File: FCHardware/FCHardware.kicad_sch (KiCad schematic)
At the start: 26 parts, among them Q1 BUT11, U1 ESC_Xrotor_65A_4in1, U2 ESP32-S3-MINI-1U, U4 TPS629203, U5 MPU-6050

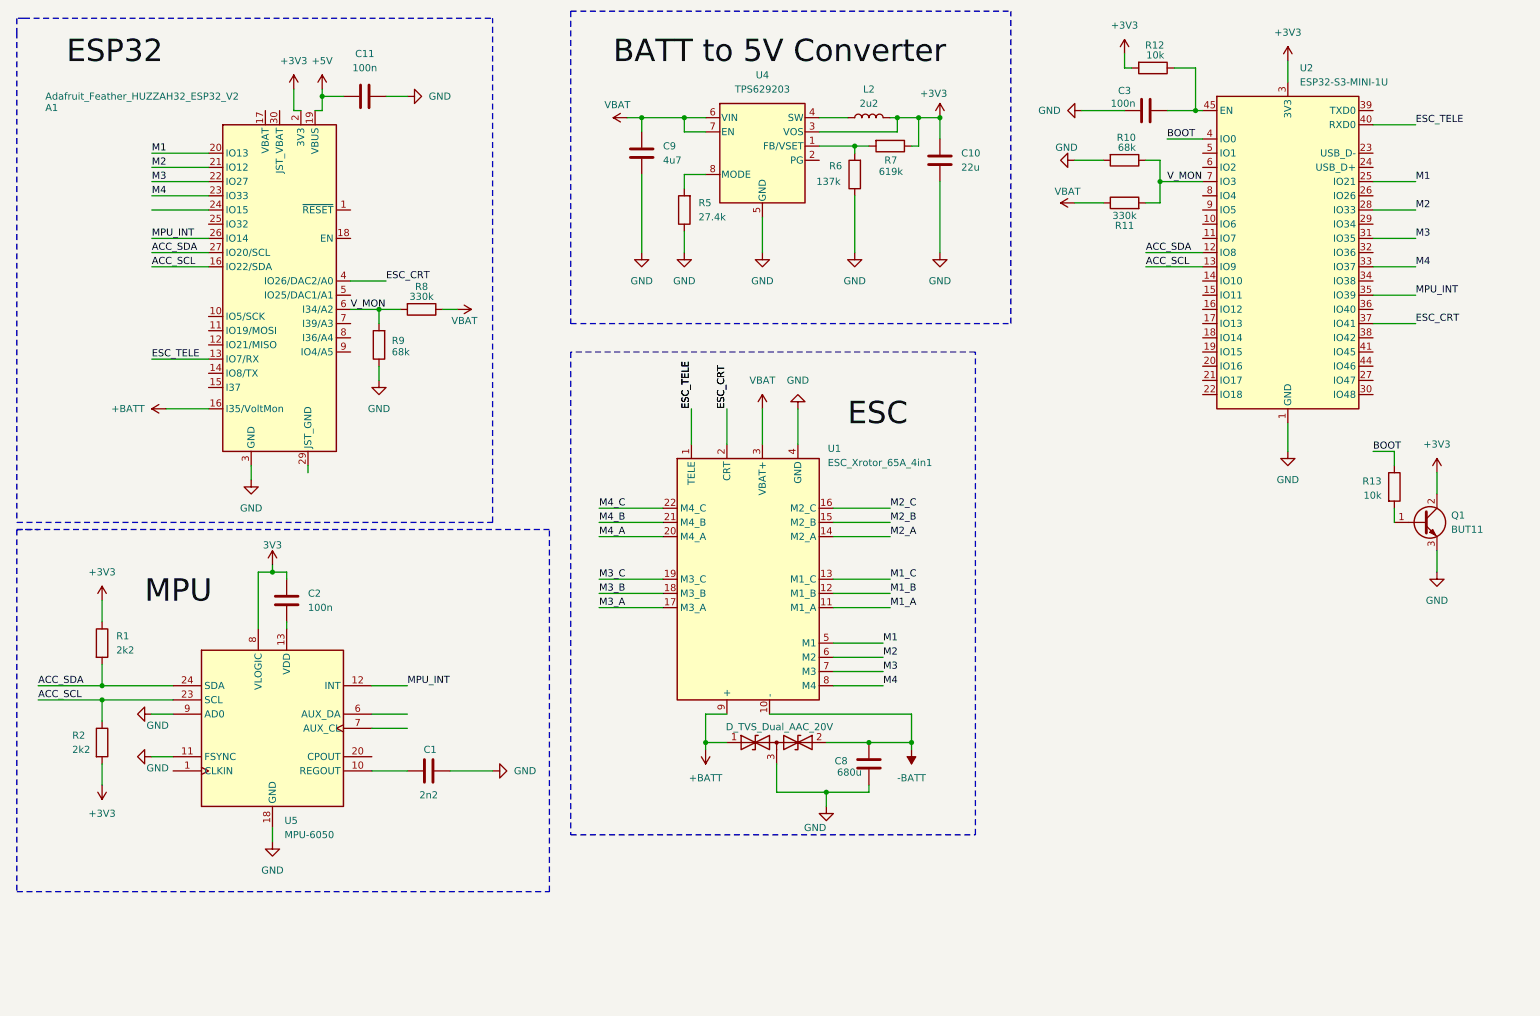
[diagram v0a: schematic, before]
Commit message: Final fixes before updating to 6S
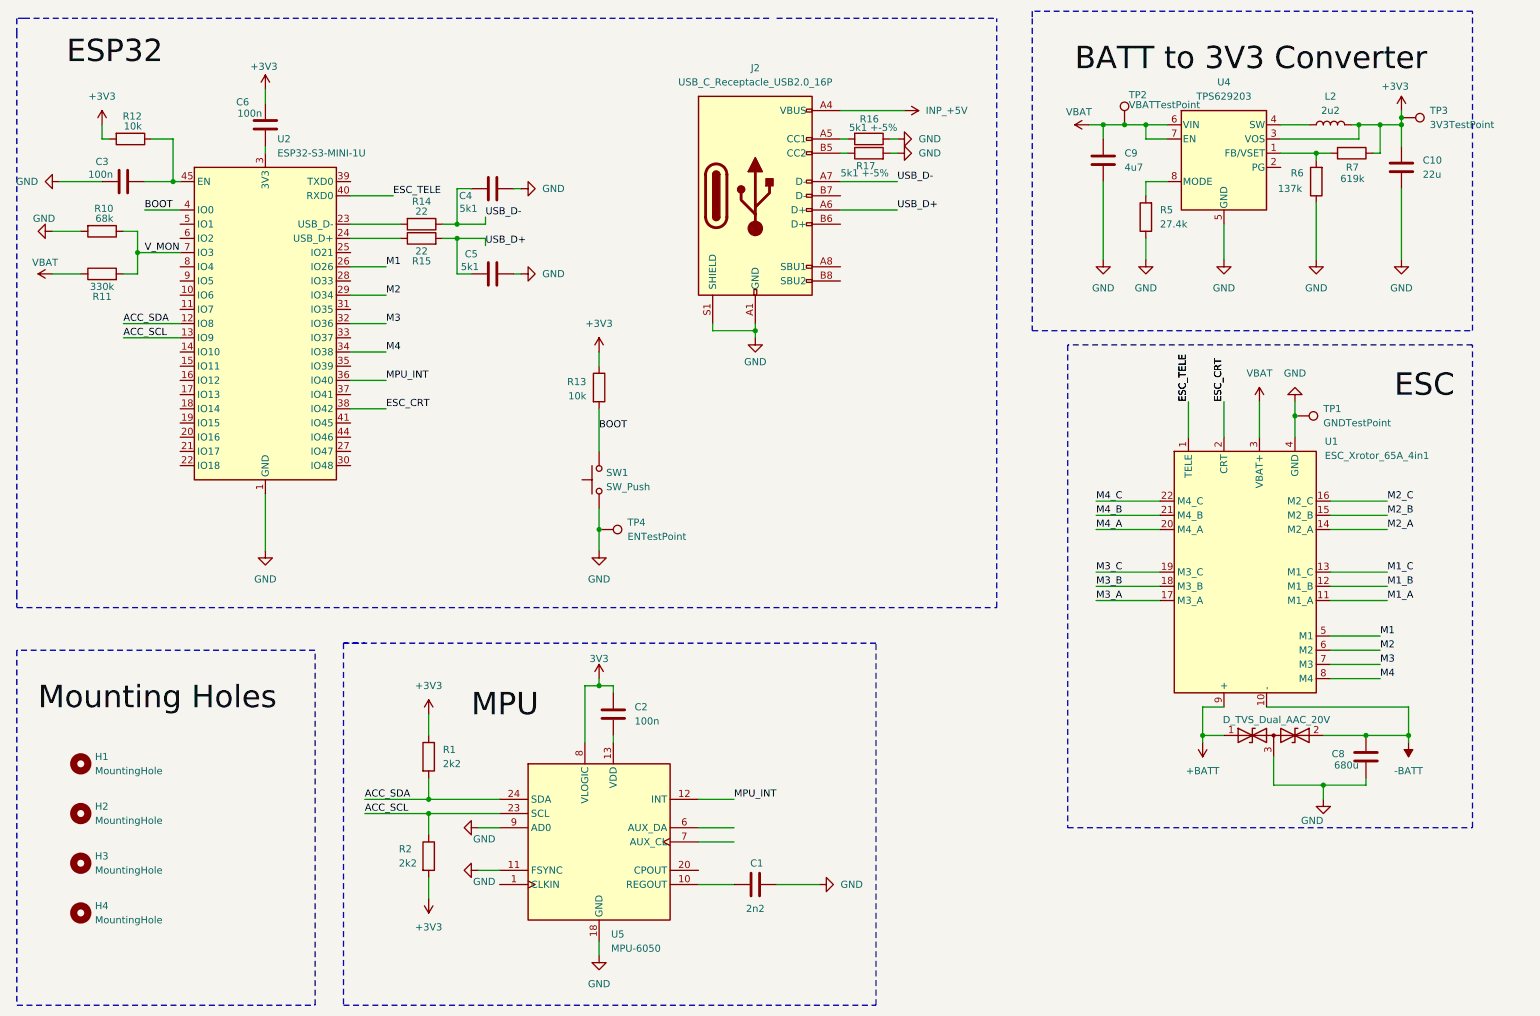
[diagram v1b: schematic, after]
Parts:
- removed A1: Adafruit_Feather_HUZZAH32_ESP32_V2, Module:Adafruit_Feather, symbol Custom_ESP32_Library:Adafruit_Feather_HUZZAH32_ESP32_v2
- removed C11: 100n, symbol Device:C
- removed Q1: BUT11, Package_TO_SOT_THT:TO-220-3_Vertical, symbol Transistor_BJT:BUT11
- removed R8: 330k, symbol Device:R
- removed R9: 68k, symbol Device:R
- added C4, C5: 5k1, symbol Device:C
- added C6: 100n, symbol Device:C
- added H1, H2, H3, H4: MountingHole, symbol Mechanical:MountingHole
- added J2: USB_C_Receptacle_USB2.0_16P, symbol Connector:USB_C_Receptacle_USB2.0_16P
- added R14, R15: 22, symbol Device:R
- added R16, R17: 5k1 +-5%, symbol Device:R
- added SW1: SW_Push, symbol Switch:SW_Push
- added TP1: GNDTestPoint, symbol Connector:TestPoint
- added TP2: VBATTestPoint, symbol Connector:TestPoint
- added TP3: 3V3TestPoint, symbol Connector:TestPoint
- added TP4: ENTestPoint, symbol Connector:TestPoint
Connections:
- net +3V3: now also R13.1, C6.2, TP3.1; no longer U2.3 (3V3)
- net BOOT: now also R13.2, SW1.2; no longer R13.1
- net ESC_CRT: now also U2.38 (IO42); no longer U2.37 (IO41)
- net GND: now also C4.2, C5.2, J2.A1 (GND), J2.A12 (GND), J2.B1 (GND), J2.B12 (GND), J2.S1 (SHIELD), R16.1, R17.2, SW1.1, TP1.1, TP4.1
- net M1: now also U2.26 (IO26); no longer U2.25 (IO21)
- net M2: now also U2.29 (IO34); no longer U2.28 (IO33)
- net M3: now also U2.32 (IO36); no longer U2.31 (IO35)
- net M4: now also U2.34 (IO38); no longer U2.33 (IO37)
- net MPU_INT: now also U2.36 (IO40); no longer U2.35 (IO39)
- net VBAT: now also TP2.1
- net at U2.23 (USB_D-): now also R14.2
- net at U2.24 (USB_D+): now also R15.1
- new net: C6.1, U2.3 (3V3)
- new net: J2.B5 (CC2), R17.1
- new net: J2.A5 (CC1), R16.2
- new net INP_+5V: J2.A4 (VBUS), J2.A9 (VBUS), J2.B4 (VBUS), J2.B9 (VBUS)
- new net USB_D+: C5.1, J2.A6 (D+), R15.2
- new net USB_D-: C4.1, J2.A7 (D-), R14.1
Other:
- moved on the sheet: C1, C10, C2, C3, C8, C9, L2, R1, R10, R11, R12, R13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
